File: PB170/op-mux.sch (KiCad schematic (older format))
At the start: 0 parts

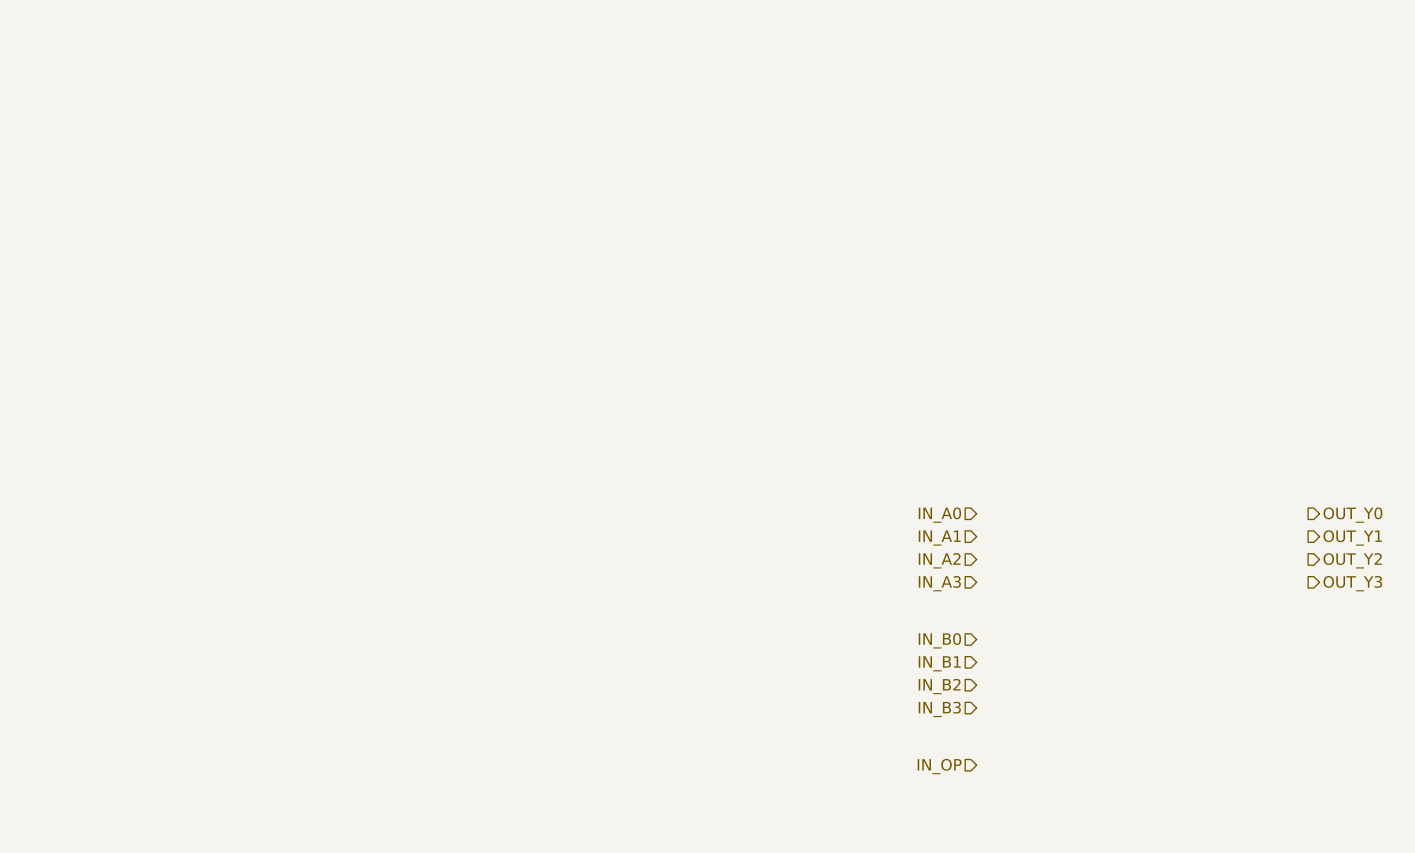
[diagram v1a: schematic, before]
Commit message: ALU finished
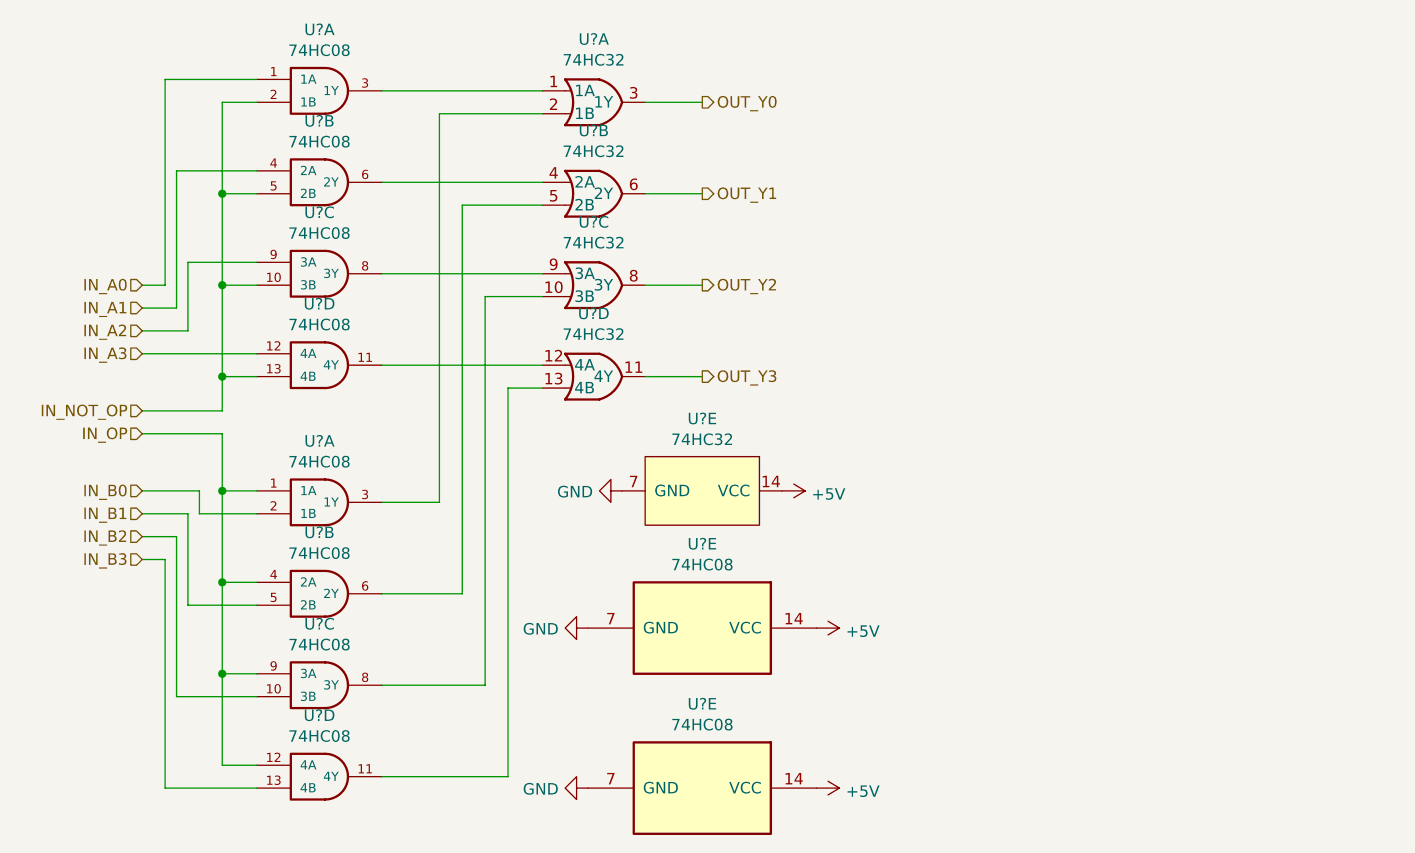
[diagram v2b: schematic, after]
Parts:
- added U? (x10): 74HC08, Housings_SOIC:SOIC-14_3.9x8.7mm_Pitch1.27mm, symbol PB170:74HC08
- added U? (x5): 74HC32, Housings_SOIC:SOIC-14_3.9x8.7mm_Pitch1.27mm, symbol PB170:74HC32
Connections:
- net IN_A0: now also U?.1 (1A)
- net IN_A1: now also U?.4 (2A)
- net IN_A2: now also U?.9 (3A)
- net IN_A3: now also U?.12 (4A)
- net IN_B0: now also U?.2 (1B)
- net IN_B1: now also U?.5 (2B)
- net IN_B2: now also U?.10 (3B)
- net IN_B3: now also U?.13 (4B)
- net IN_OP: now also U?.1 (1A), U?.12 (4A), U?.4 (2A), U?.9 (3A)
- net OUT_Y0: now also U?.3 (1Y)
- net OUT_Y1: now also U?.6 (2Y)
- net OUT_Y2: now also U?.8 (3Y)
- net OUT_Y3: now also U?.11 (4Y)
- new net: U?.1 (1A), U?.3 (1Y)
- new net: U?.4 (2A), U?.6 (2Y)
- new net: U?.8 (3Y), U?.9 (3A)
- new net: U?.11 (4Y), U?.12 (4A)
- new net: U?.2 (1B), U?.3 (1Y)
- new net: U?.5 (2B), U?.6 (2Y)
- new net: U?.10 (3B), U?.8 (3Y)
- new net: U?.11 (4Y), U?.13 (4B)
- new net +5V: U?.14 (VCC), U?.14 (VCC), U?.14 (VCC)
- new net GND: U?.7 (GND), U?.7 (GND), U?.7 (GND)
- new net IN_NOT_OP: U?.10 (3B), U?.13 (4B), U?.2 (1B), U?.5 (2B)
